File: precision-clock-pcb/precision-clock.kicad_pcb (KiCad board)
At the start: 4 copper layers, 500 x 34 mm, 150 parts, among them J1 USB_C_Receptacle_USB2.0_14P, J2 TC2050, J3 ANT, Q1 SFH320, Q10 BSS138, Q11 BSS138, Q12 BSS138, Q13 BSS138, Q14 BSS138, Q15 BSS138, Q16 BSS138, Q2 SFH320, Q3 BSS83P, Q4 BSS138, Q5 BSS138, Q6 BSS138, Q7 BSS138, Q8 BSS138, Q9 BSS138, SW1 BOOTSEL, SW2 RESET, SW3 BUTTON, SW4 BUTTON, U1 NCP1117-3.3_SOT223, U10 CD74HCT238M96, U2 USBLC6-2P6, U3 W25Q128JVS, U4 RP2350_80QFN, U5 PA1616S, U6 DS3232M, U7 CD74HCT238M96, U8 SN74ABT244ADW, U9 SN74ABT244ADW, Y1 ABM8-272-T3

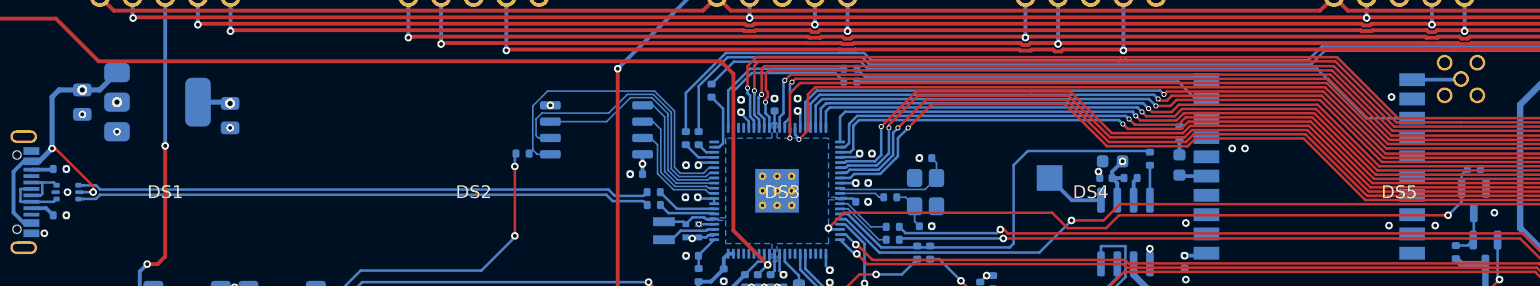
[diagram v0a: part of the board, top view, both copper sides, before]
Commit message: BOM, CSV, and STEP exports
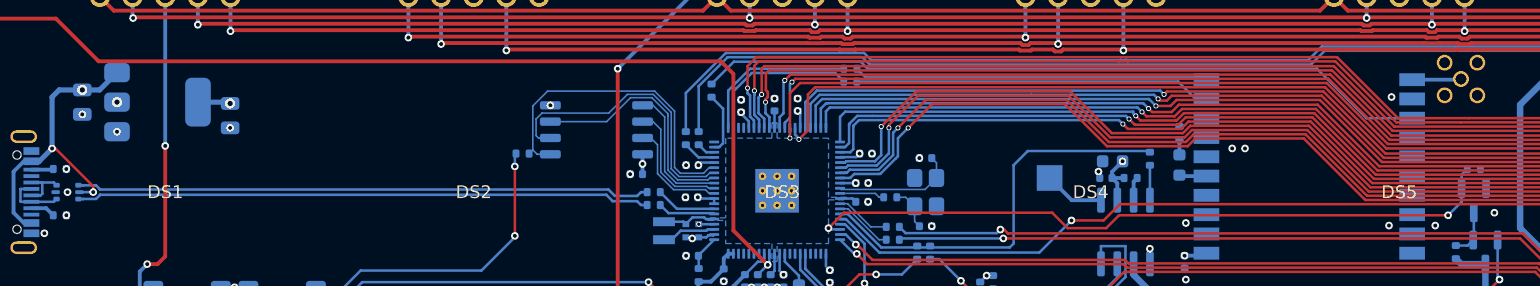
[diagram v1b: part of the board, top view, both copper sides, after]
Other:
- board text added: "Ordering notes: Specify stackup so that In2.Cu is directly above B.Cu to ensure proper grounding of impedance controlled traces Use JLC 4 layer controlled stackup JLC04161H-7628 (default stackup) Min via size 0.25/0.4mm, order with vias epoxy filled and capped"
- board text removed: "Ordering notes: 4 layers, 1oz outer 1oz inner. Specify stackup so that In2.Cu is directly above B.Cu to ensure proper grounding of impedance controlled traces Use JLC 4 layer controlled stackup JLC041611-7628 Min via size 0.25/0.4mm, order with vias epoxy filled and capped Remove Mark and please order it in something other than Green or Yellow"
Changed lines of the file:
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@@
 	(footprint "Resistor_SMD:R_0402_1005Metric"
 		(layer "B.Cu")
-		(at 69.01 46)
+		(at 69 46)
 		(descr "Resistor SMD 0402 (1005 Metric), square (rectangular) end terminal, IPC-7351 nominal, (Body size source: IPC-SM-782 page 72, https://www.pcb-3d.com/wordpress/wp-content/uploads/ipc-sm-782a_amendment_1_and_2.pdf), generated with kicad-footprint-generator")
 		(tags "resistor")
@@
 			(size 0.6 0.6)
 			(drill 0.25)
-			(layers "F&B.Cu" "B.Mask")
+			(layers "*.Cu" "B.Mask")
 			(remove_unused_layers no)
 			(net 2 "GND")
@@
 			(size 0.6 0.6)
 			(drill 0.25)
-			(layers "F&B.Cu" "B.Mask")
+			(layers "*.Cu" "B.Mask")
 			(remove_unused_layers no)
 			(net 2 "GND")
@@
 			(size 0.6 0.6)
 			(drill 0.25)
-			(layers "F&B.Cu" "B.Mask")
+			(layers "*.Cu" "B.Mask")
 			(remove_unused_layers no)
 			(net 2 "GND")
@@
 			(size 0.6 0.6)
 			(drill 0.25)
-			(layers "F&B.Cu" "B.Mask")
+			(layers "*.Cu" "B.Mask")
 			(remove_unused_layers no)
 			(net 2 "GND")
@@
 			(size 0.6 0.6)
 			(drill 0.25)
-			(layers "F&B.Cu" "B.Mask")
+			(layers "*.Cu" "B.Mask")
 			(remove_unused_layers no)
 			(net 2 "GND")
@@
 			(size 0.6 0.6)
 			(drill 0.25)
-			(layers "F&B.Cu" "B.Mask")
+			(layers "*.Cu" "B.Mask")
 			(remove_unused_layers no)
 			(net 2 "GND")
@@
 			(size 0.6 0.6)
 			(drill 0.25)
-			(layers "F&B.Cu" "B.Mask")
+			(layers "*.Cu" "B.Mask")
 			(remove_unused_layers no)
 			(net 2 "GND")
@@
 			(size 0.6 0.6)
 			(drill 0.25)
-			(layers "F&B.Cu" "B.Mask")
+			(layers "*.Cu" "B.Mask")
 			(remove_unused_layers no)
 			(net 2 "GND")
@@
 			(size 0.6 0.6)
 			(drill 0.25)
-			(layers "F&B.Cu" "B.Mask")
+			(layers "*.Cu" "B.Mask")
 			(remove_unused_layers no)
 			(net 2 "GND")
@@
 			(size 2.775 2.775)
 			(drill 1.85)
-			(layers "F&B.Cu" "*.Mask")
+			(layers "*.Cu" "*.Mask")
 			(remove_unused_layers no)
 			(net 1 "+BATT")
@@
 			(size 2.775 2.775)
 			(drill 1.85)
-			(layers "F&B.Cu" "*.Mask")
+			(layers "*.Cu" "*.Mask")
 			(remove_unused_layers no)
 			(net 1 "+BATT")
@@
 			(drill oval 0.6 1.4)
 			(property pad_prop_heatsink)
-			(layers "F&B.Cu" "*.Mask")
+			(layers "*.Cu" "*.Mask")
 			(remove_unused_layers no)
 			(net 2 "GND")
@@
 			(drill oval 0.6 1.7)
 			(property pad_prop_heatsink)
-			(layers "F&B.Cu" "*.Mask")
+			(layers "*.Cu" "*.Mask")
 			(remove_unused_layers no)
 			(net 2 "GND")
@@
 			(drill oval 0.6 1.4)
 			(property pad_prop_heatsink)
-			(layers "F&B.Cu" "*.Mask")
+			(layers "*.Cu" "*.Mask")
 			(remove_unused_layers no)
 			(net 2 "GND")
@@
 			(drill oval 0.6 1.7)
 			(property pad_prop_heatsink)
-			(layers "F&B.Cu" "*.Mask")
+			(layers "*.Cu" "*.Mask")
 			(remove_unused_layers no)
 			(net 2 "GND")
@@
 			(size 1.24 1.24)
 			(drill 0.84)
-			(layers "F&B.Cu" "*.Mask")
+			(layers "*.Cu" "*.Mask")
 			(remove_unused_layers no)
 			(net 60 "/GPS/ANT")
@@
 			(size 1.24 1.24)
 			(drill 0.84)
-			(layers "F&B.Cu" "*.Mask")
+			(layers "*.Cu" "*.Mask")
 			(remove_unused_layers no)
 			(net 2 "GND")
@@
 			(size 1.24 1.24)
 			(drill 0.84)
-			(layers "F&B.Cu" "*.Mask")
+			(layers "*.Cu" "*.Mask")
 			(remove_unused_layers no)
 			(net 2 "GND")
@@
 			(size 1.24 1.24)
 			(drill 0.84)
-			(layers "F&B.Cu" "*.Mask")
+			(layers "*.Cu" "*.Mask")
 			(remove_unused_layers no)
 			(net 2 "GND")
@@
 			(size 1.24 1.24)
 			(drill 0.84)
-			(layers "F&B.Cu" "*.Mask")
+			(layers "*.Cu" "*.Mask")
 			(remove_unused_layers no)
 			(net 2 "GND")
@@
 		)
 	)
-	(gr_text "Ordering notes:\n4 layers, 1oz outer 1oz inner. Specify stackup so that In2.Cu is directly above B.Cu to ensure proper grounding of impedance controlled traces\nUse JLC 4 layer controlled stackup JLC041611-7628\nMin via size 0.25/0.4mm, order with vias epoxy filled and capped\nRemove Mark and please order it in something other than Green or Yellow"
+	(gr_text "Ordering notes:\nSpecify stackup so that In2.Cu is directly above B.Cu to ensure proper grounding of impedance controlled traces\nUse JLC 4 layer controlled stackup JLC04161H-7628 (default stackup)\nMin via size 0.25/0.4mm, order with vias epoxy filled and capped"
 		(at 13.4 71.8 0)
 		(layer "F.Fab")
@@
 	)
 	(segment
-		(start 128 36.25)
-		(end 131.75 36.25)
-		(width 0.286258)
+		(start 131.75 36.25)
+		(end 131.8 36.2)
+		(width 0.295402)
 		(layer "B.Cu")
 		(net 60)
 	)
 	(segment
-		(start 131.75 36.25)
-		(end 131.8 36.2)
-		(width 0.286258)
+		(start 128 36.25)
+		(end 131.75 36.25)
+		(width 0.295402)
 		(layer "B.Cu")
 		(net 60)
@@
 	)
 	(segment
-		(start 65.483379 44.798705)
-		(end 25.927695 44.798705)
-		(width 0.19939)
+		(start 67.713453 45.296546)
+		(end 65.984274 45.296546)
+		(width 0.203708)
 		(layer "B.Cu")
 		(net 85)
 	)
 	(segment
-		(start 24.634806 44.472305)
-		(end 24.625001 44.4625)
-		(width 0.19939)
+		(start 68.009999 45)
+		(end 67.713453 45.296546)
+		(width 0.203708)
 		(layer "B.Cu")
 		(net 85)
 	)
 	(segment
-		(start 24.625001 44.4625)
-		(end 24.25 44.4625)
-		(width 0.19939)
+		(start 25.929854 44.780527)
+		(end 25.619473 44.470146)
+		(width 0.203708)
 		(layer "B.Cu")
 		(net 85)
 	)
 	(segment
-		(start 25.618579 44.472305)
-		(end 24.634806 44.472305)
-		(width 0.19939)
+		(start 68.49 45)
+		(end 68.009999 45)
+		(width 0.203708)
 		(layer "B.Cu")
 		(net 85)
 	)
 	(segment
-		(start 68.49 45)
-		(end 68.196296 45.293704)
-		(width 0.19939)
+		(start 25.619473 44.470146)
+		(end 24.632647 44.470146)
+		(width 0.203708)
+		(layer "B.Cu")
+		(net 85)
+	)
+	(segment
+		(start 65.984274 45.296546)
+		(end 65.484274 44.796546)
+		(width 0.203708)
 		(layer "B.Cu")
 		(net 85)
 	)
 	(segment
-		(start 25.927695 44.798705)
-		(end 25.927695 44.781421)
-		(width 0.19939)
+		(start 25.929854 44.796546)
+		(end 25.929854 44.780527)
+		(width 0.203708)
 		(layer "B.Cu")
 		(net 85)
 	)
 	(segment
-		(start 65.978378 45.293704)
-		(end 65.483379 44.798705)
-		(width 0.19939)
+		(start 24.625001 44.4625)
+		(end 24.25 44.4625)
+		(width 0.203708)
 		(layer "B.Cu")
 		(net 85)
 	)
 	(segment
-		(start 25.927695 44.781421)
-		(end 25.618579 44.472305)
-		(width 0.19939)
+		(start 65.484274 44.796546)
+		(end 25.929854 44.796546)
+		(width 0.203708)
 		(layer "B.Cu")
 		(net 85)
 	)
 	(segment
-		(start 68.196296 45.293704)
-		(end 65.978378 45.293704)
-		(width 0.19939)
+		(start 24.632647 44.470146)
+		(end 24.625001 44.4625)
+		(width 0.203708)
 		(layer "B.Cu")
 		(net 85)
 	)
 	(segment
-		(start 65.811622 45.696296)
-		(end 65.316621 45.201295)
-		(width 0.19939)
+		(start 65.815726 45.703454)
+		(end 65.315726 45.203454)
+		(width 0.203708)
 		(layer "B.Cu")
 		(net 86)
 	)
 	(segment
-		(start 24.625001 45.5375)
-		(end 24.25 45.5375)
-		(width 0.19939)
+		(start 67.713453 45.703454)
+		(end 65.815726 45.703454)
+		(width 0.203708)
 		(layer "B.Cu")
 		(net 86)
 	)
 	(segment
-		(start 25.927695 45.201295)
-		(end 25.927695 45.218579)
-		(width 0.19939)
+		(start 65.315726 45.203454)
+		(end 25.929854 45.203454)
+		(width 0.203708)
 		(layer "B.Cu")
 		(net 86)
 	)
 	(segment
-		(start 68.196296 45.696296)
-		(end 65.811622 45.696296)
-		(width 0.19939)
+		(start 25.929854 45.203454)
+		(end 25.929854 45.219473)
+		(width 0.203708)
 		(layer "B.Cu")
 		(net 86)
 	)
 	(segment
-		(start 25.927695 45.218579)
-		(end 25.618579 45.527695)
-		(width 0.19939)
+		(start 25.929854 45.219473)
+		(end 25.619473 45.529854)
+		(width 0.203708)
 		(layer "B.Cu")
 		(net 86)
 	)
 	(segment
-		(start 24.634806 45.527695)
-		(end 24.625001 45.5375)
-		(width 0.19939)
+		(start 25.619473 45.529854)
+		(end 24.632647 45.529854)
+		(width 0.203708)
 		(layer "B.Cu")
 		(net 86)
 	)
 	(segment
-		(start 68.5 46)
-		(end 68.196296 45.696296)
-		(width 0.19939)
+		(start 68.49 46)
+		(end 68.009999 46)
+		(width 0.203708)
 		(layer "B.Cu")
 		(net 86)
 	)
 	(segment
-		(start 25.618579 45.527695)
-		(end 24.634806 45.527695)
-		(width 0.19939)
+		(start 68.009999 46)
+		(end 67.713453 45.703454)
+		(width 0.203708)
 		(layer "B.Cu")
 		(net 86)
 	)
 	(segment
-		(start 65.316621 45.201295)
-		(end 25.927695 45.201295)
-		(width 0.19939)
+		(start 24.632647 45.529854)
+		(end 24.625001 45.5375)
+		(width 0.203708)
 		(layer "B.Cu")
 		(net 86)
 	)
 	(segment
-		(start 70.1545 46.6345)
-		(end 69.52 46)
-		(width 0.2)
+		(start 24.625001 45.5375)
+		(end 24.25 45.5375)
+		(width 0.203708)
 		(layer "B.Cu")
-		(net 87)
+		(net 86)
 	)
 	(segment
@@
 		(width 0.2)
 		(layer "B.Cu")
+		(net 87)
+	)
+	(segment
+		(start 69.52 46)
+		(end 69.51 46)
+		(width 0.2)
+		(layer "B.Cu")
+		(net 87)
+	)
+	(segment
+		(start 70.1545 46.6345)
+		(end 69.52 46)
+		(width 0.2)
+		(layer "B.Cu")
